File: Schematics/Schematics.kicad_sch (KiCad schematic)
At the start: 8 parts, among them Q1 BC547, U1 CY8C5888LTI-LP09, U2 LM78L05, U3 Adafruit_BNO08x

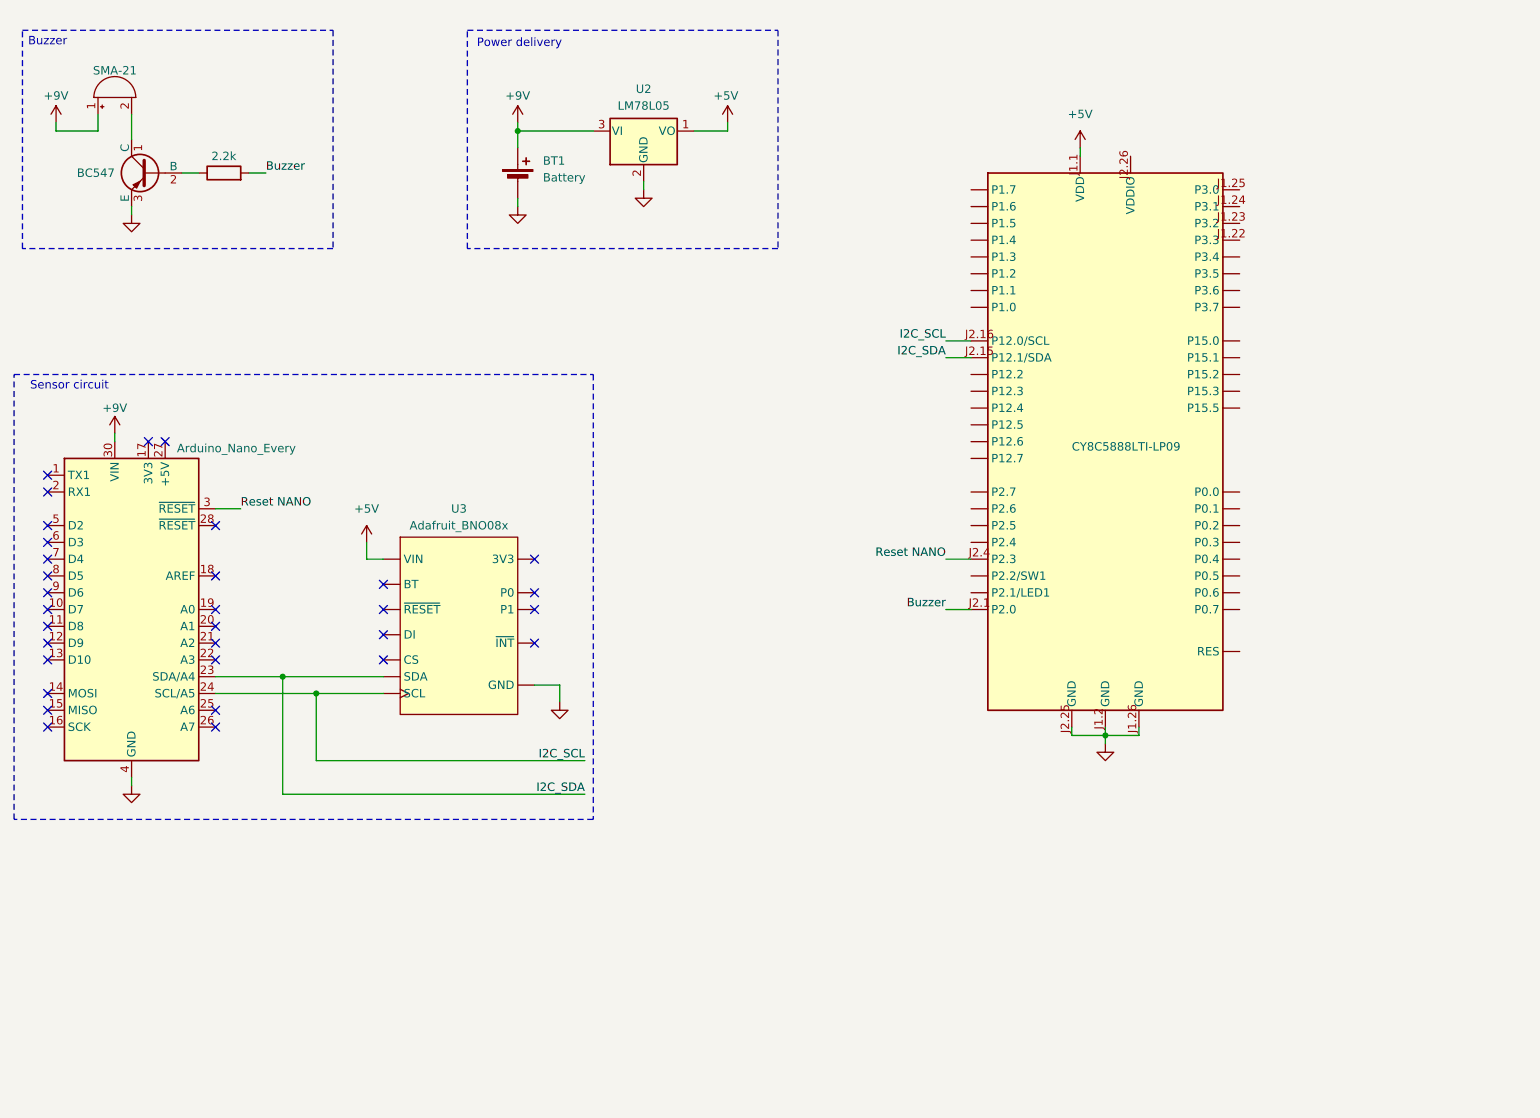
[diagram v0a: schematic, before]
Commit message: opdaterede schematics
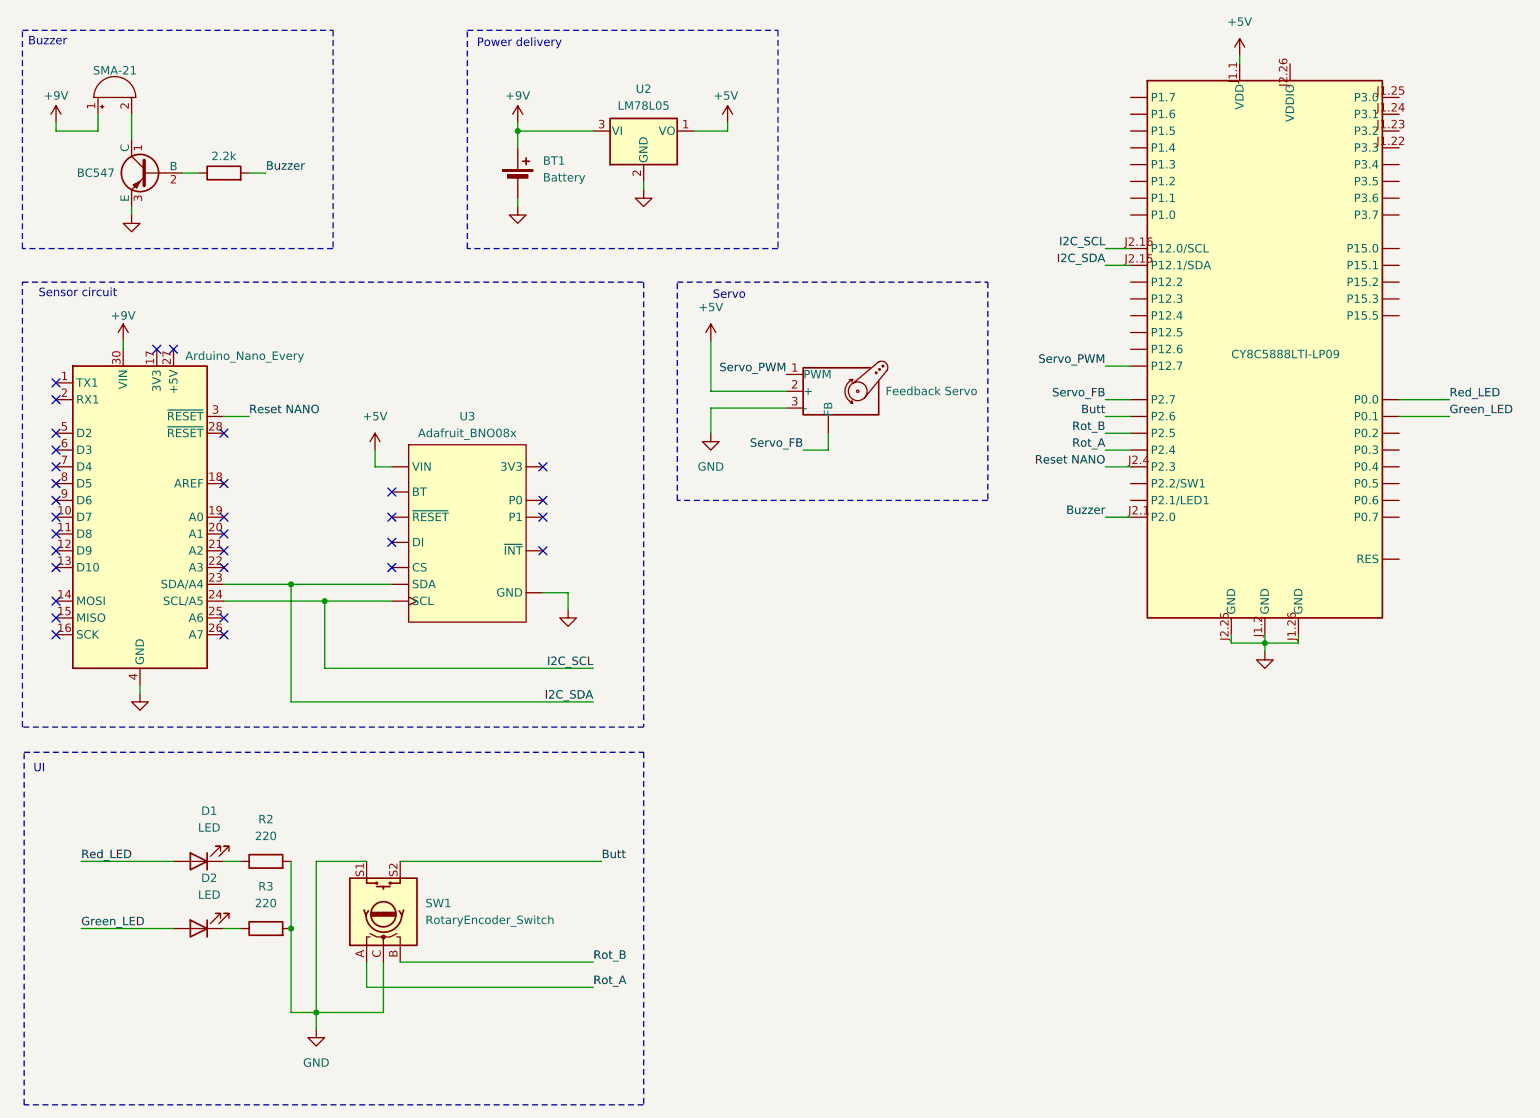
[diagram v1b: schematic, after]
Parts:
- added D1, D2: LED, symbol Device:LED
- added M1: Feedback Servo, symbol Motor:Motor_Servo
- added R2, R3: 220, symbol Device:R
- added SW1: RotaryEncoder_Switch, symbol Device:RotaryEncoder_Switch
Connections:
- net +5V: now also M1.2 (+)
- net GND: now also M1.3 (-), R2.2, R3.2, SW1.C, SW1.S1
- net Servo_PWM: now reaches U1. (RES)
- net Servo_PWM: now also M1.1 (PWM)
- new net: D2.1 (K), R3.1
- new net: D1.1 (K), R2.1
- new net Butt: SW1.S2, U1. (RES)
- new net Green_LED: D2.2 (A), U1. (RES)
- new net Red_LED: D1.2 (A), U1. (RES)
- new net Rot_A: SW1.A, U1. (RES)
- new net Rot_B: SW1.B, U1. (RES)
- new net Servo_FB: M1. (FB), U1. (RES)
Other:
- note added: "Servo"
- note added: "UI"
- moved on the sheet: U3
